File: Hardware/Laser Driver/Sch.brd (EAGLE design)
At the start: 160 x 100 mm, 33 parts, among them IC1 LMH6645MF

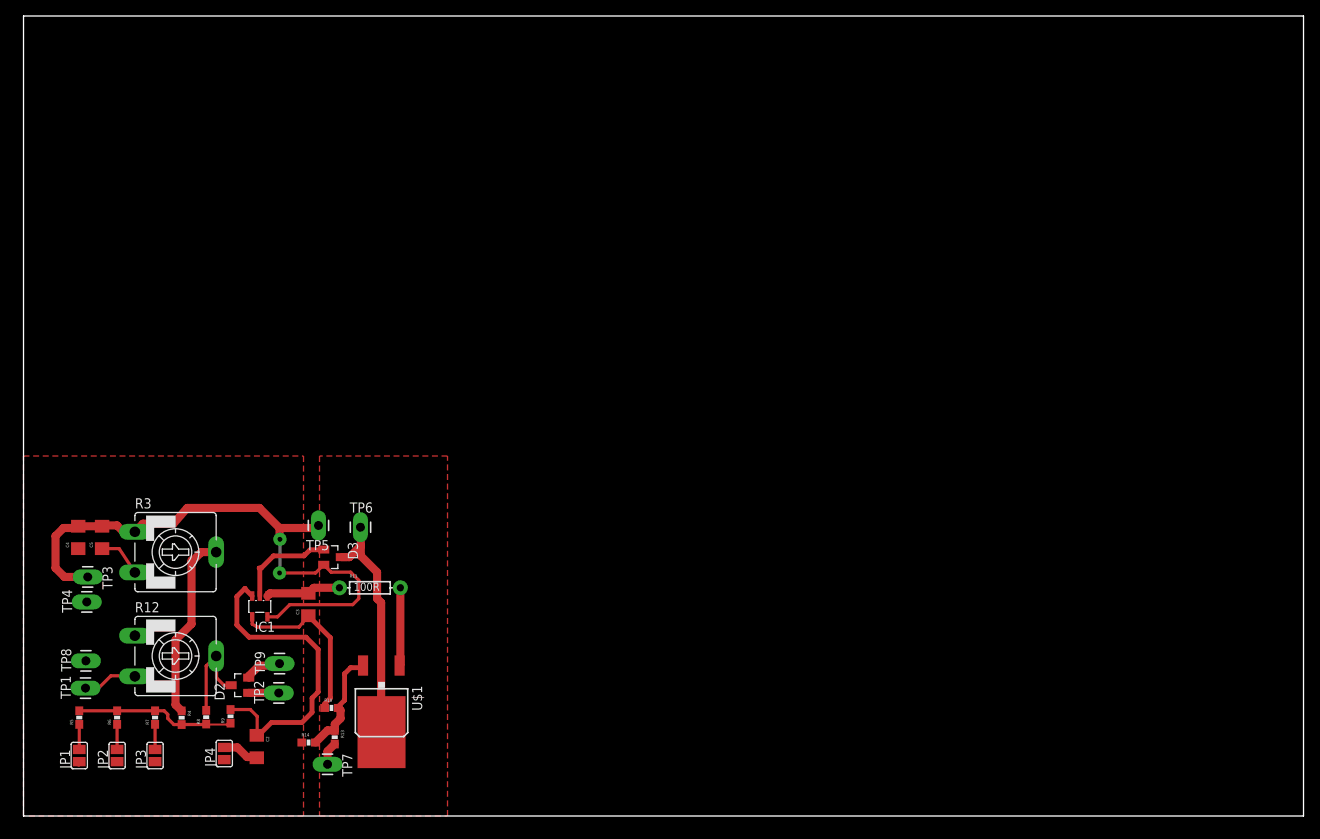
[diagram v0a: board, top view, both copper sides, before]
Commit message: Added hardware and software files
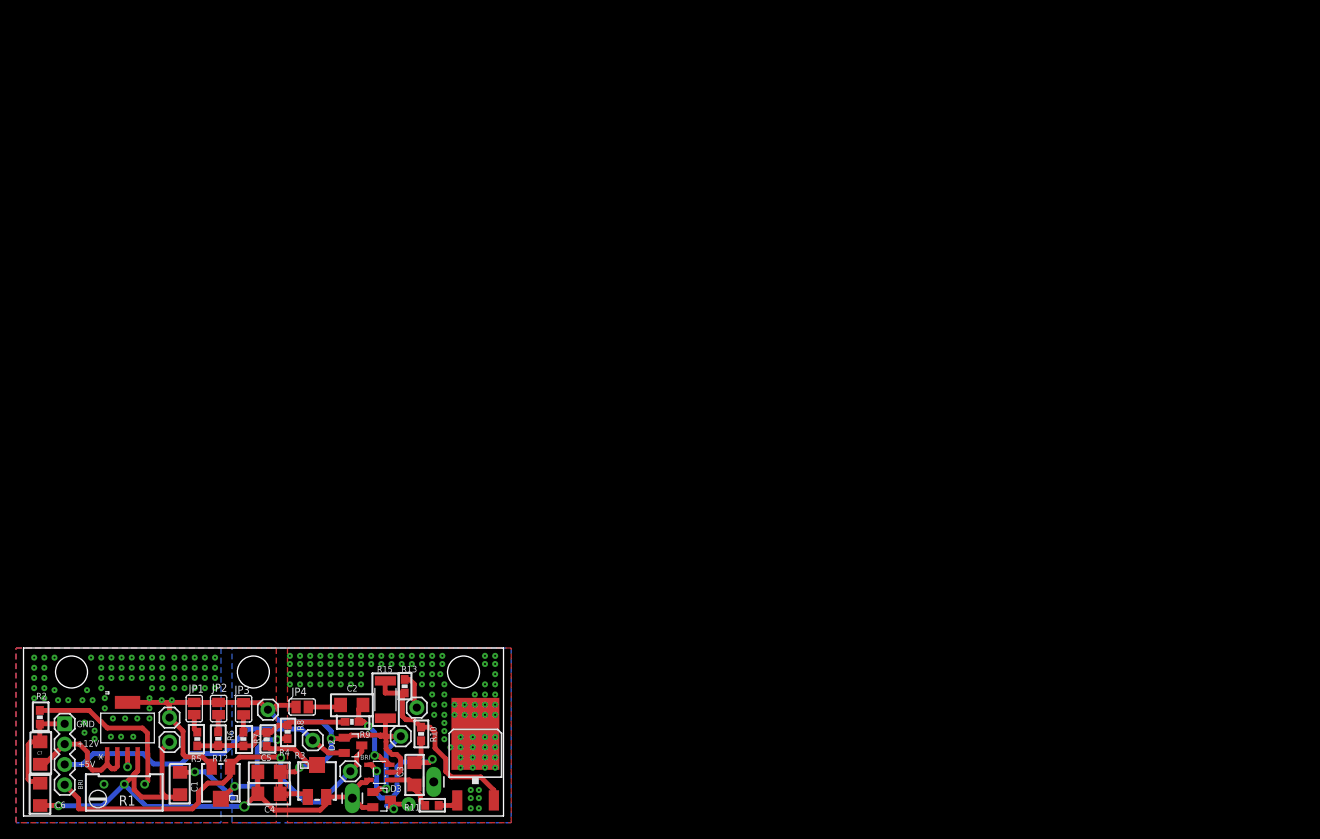
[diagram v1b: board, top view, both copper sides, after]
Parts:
- removed R14: 1R, SparkFun-Passives:0603-RES
- added C1: 100n, SparkFun-Passives:1206
- added C6: 15u, SparkFun-Passives:1206
- added C7: 10u, SparkFun-Passives:1206
- added JP6: (no value), SparkFun-Connectors:1X04
- added R1: 5k, resistor:RTRIM64W
- added R15: 1R, EagleParts:RESC5025X71N
- added R2: 240R, SparkFun-Passives:0603-RES
- added U1: TL1963ADCQR, EagleParts:SOT127P700X180-6N
- C5: value 47u -> 15u
- R11: device SparkFun-Passives:AXIAL-0.3 -> resistor:R0603
- R12, R3: device pot:CA9V -> resistor:RTRIM5X
- R4: value (none) -> 22k
- TP1, TP2, TP3, TP4, TP7, TP8, TP9: device SparkFun-Connectors:1X01_LONGPAD -> SparkFun-Connectors:1X01
- moved C4 39.9 mm to (30.7, 2.78), turned to 180 degrees
- moved C5 36.0 mm to (30.7, 5.52), turned to 180 degrees
- moved TP1 34.7 mm to (40.9, 5.59)
- moved TP5 34.4 mm to (41.1, 2.23)
- moved R3 33.6 mm to (36.7, 4.38), turned to 0 degrees
- moved TP6 33.1 mm to (51.3, 4.27)
- moved D3 30.9 mm to (44.8, 2.05)
- moved R11 28.3 mm to (51.1, 1.32)
- moved TP4 26.3 mm to (30.6, 13.3)
- moved IC1 25.6 mm to (44.5, 5.46), turned to 90 degrees
- moved C3 25.0 mm to (48.9, 5.27), turned to 270 degrees
- moved TP3 23.0 mm to (18.3, 9.25)
- moved R12 16.8 mm to (24.7, 4.15), turned to 180 degrees
- moved TP2 16.2 mm to (47.2, 9.96)
- moved D2 16.0 mm to (41.2, 8.83), turned to 270 degrees
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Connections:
- removed net N$1: R12.E, TP1.1
- new net +12V: C7.1, JP6.2, U1.1, U1.2
- new net BRIGHTNESS: D2.3, JP6.4, R12.1, TP1.1
- new net N$16: R1.1, R2.2, U1.5
- net +5V: now also JP6.3
- net GNDA: now also C6.2, C7.2, JP6.1, R12.3, R15.2, R2.1, R3.1, U1.3, U1.6; no longer R12.A, R14.1, R3.E
- net N$11: now also R11.1; no longer R11.P$1
- net N$12: now also R11.2; no longer R11.P$2
- net N$14: now also C1.1
- net N$15: now also R15.1; no longer R14.2
- net N$2: now also R12.2; no longer D2.3, R12.S
- net N$3: now also R3.2; no longer R3.S
- net VCC: now also C1.2, C6.1, R1.2, R3.3, U1.4; no longer R3.A
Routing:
- net GNDA: track 22.8 -> 101.7 mm, vias 0 -> 83
- net BRIGHTNESS: track 0.00 -> 51.3 mm, vias 0 -> 1
- net +5V: track 4.74 -> 39.0 mm
- net N$9: track 40.1 -> 10.2 mm, vias 0 -> 2
- net N$16: track 0.00 -> 21.2 mm
- net N$14: track 29.7 -> 12.9 mm, vias 0 -> 109
- net +12V: track 0.00 -> 16.6 mm
- net N$3: track 23.6 -> 7.27 mm
- net N$15: track 13.6 -> 26.0 mm
- net N$12: track 9.76 -> 2.58 mm
- net N$1: track 6.84 -> 0.00 mm
- net VCC: track 77.6 -> 74.1 mm
- net N$11: track 9.43 -> 6.46 mm
- net N$17: track 2.91 -> 4.83 mm
- net N$2: track 12.3 -> 14.2 mm, vias 0 -> 2
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- added copper zone on layer 16, net GNDA
- added copper zone on layer 16, net N$14
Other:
- board size 160 x 100 mm -> 60 x 21 mm
- board text added: "+12V"
- board text added: "+5V"
- board text added: "BRI"
- board text added: "GND"
